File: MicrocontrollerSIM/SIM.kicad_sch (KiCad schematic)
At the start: 104 parts, among them J1 Conn_01x15_Socket, J2 JAE_SIM_Card_SF72S006, J3 Micro_SD_Card_Det_Hirose_DM3AT, J6 Conn_01x04_Pin, J7 Conn_Coaxial, Q1 BC848, Q2 BC848, Q3 BC848, Q4 BC848, Q5 NPN, SW1 SW_Push, SW3 SW_Push, U1 AMS1117-3.3, U2 TXS0104EPW, U3 EC200UCNAA-N05-SGNSA, U4 MIC29302AWD, U6 RT9193-18GB, U7 STM32F411CEUx, Y1 25MHz, Y2 32.768KHz

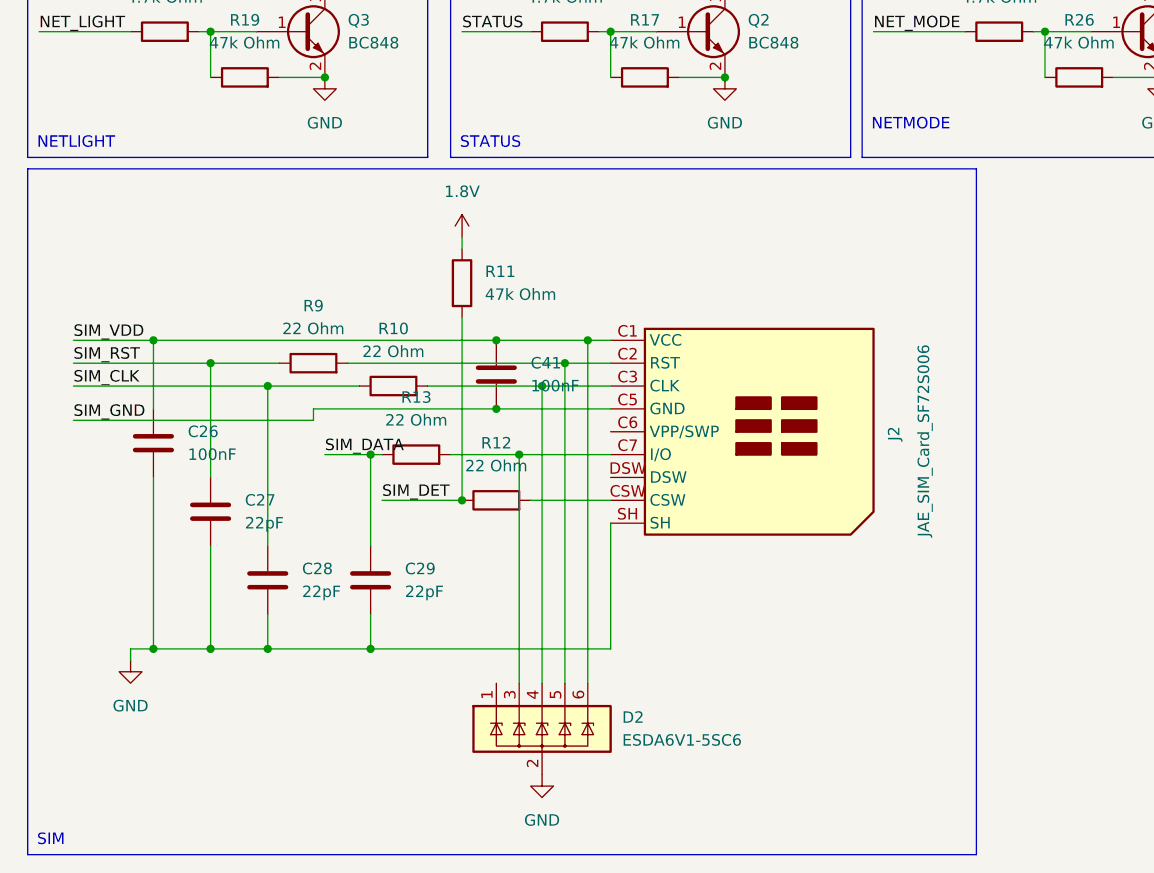
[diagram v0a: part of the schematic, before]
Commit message: sim change
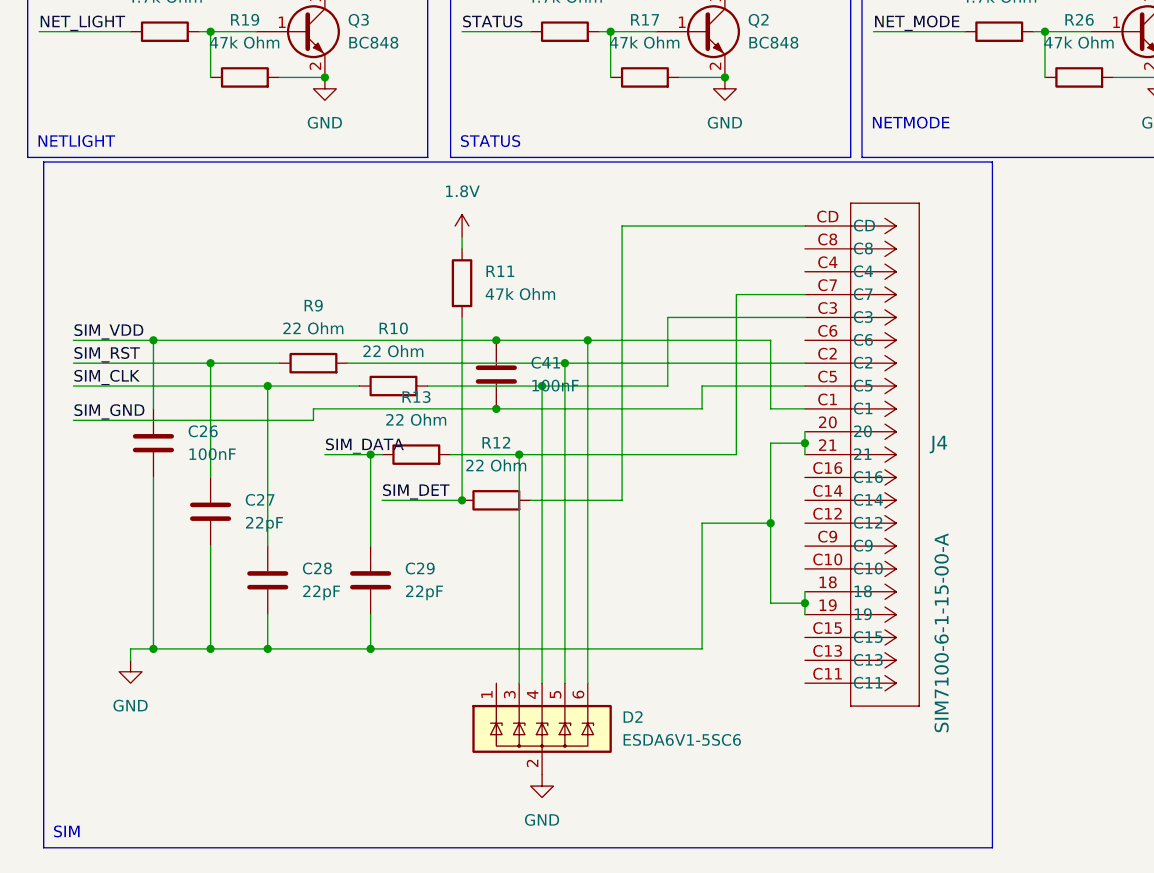
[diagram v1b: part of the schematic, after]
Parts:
- removed J2: JAE_SIM_Card_SF72S006, Connector_JAE:JAE_SIM_Card_SF72S006, symbol Connector:JAE_SIM_Card_SF72S006
- added J4: SIM7100-6-1-15-00-A, CONN21_-6-1-15-00-A_GCT, symbol SIM7100-6-1-15-00-A:SIM7100-6-1-15-00-A
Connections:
- net GND: now also J4.18, J4.19, J4.20, J4.21
- net SIM_GND: now also J4.C5
- net SIM_VDD: now also J4.C1
- net at D2.3 (IO2), R13.2: now also J4.C7
- net at D2.5 (IO4), R9.2: now also J4.C2
- net at D2.4 (IO3), R10.2: now also J4.C3
- net at R12.2: now also J4.CD
